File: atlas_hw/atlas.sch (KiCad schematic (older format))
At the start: 200 parts, among them J1 USB_C_Receptacle_USB2.0, J10 PSP_LCD, J2 DEBUG_STM, J3 PSP_TOUCH, J4 DEBUG_NRF, J5 CELL_THERM, J6 CELL_BARE, J7 AUX_THERM, J8 Micro_SD_Card_Det, J9 PSP_LCD_BL, Q1 Q_NMOS_DGS, Q2 Q_NMOS_DGS, Q3 Q_NMOS_DGS, Q4 Q_NMOS_DGS, Q5 Q_NMOS_DGS, SW1 SReset, SW2 Power, SW3 ResetSTM, SW4 ResetNRF, U1 STM32H723VITx, U10 BQ25611D, U11 STM6601CA2BDM6F, U12 BGA725L6, U13 LSF0108, U14 NPP600SNADJ, U15 TPS61073, U16 PAM2841, U17 NX3L1T3157, U2 W957A8MFYA5I, U3 MCP1811B, U4 TLV62569DBV, U5 nRF52810-QCxx, U6 LC709203F, U7 Teseo-LIV3F, U8 MS5637, U9 MC6470, Y1 16M, Y2 32k, Y3 32M, Y4 32k

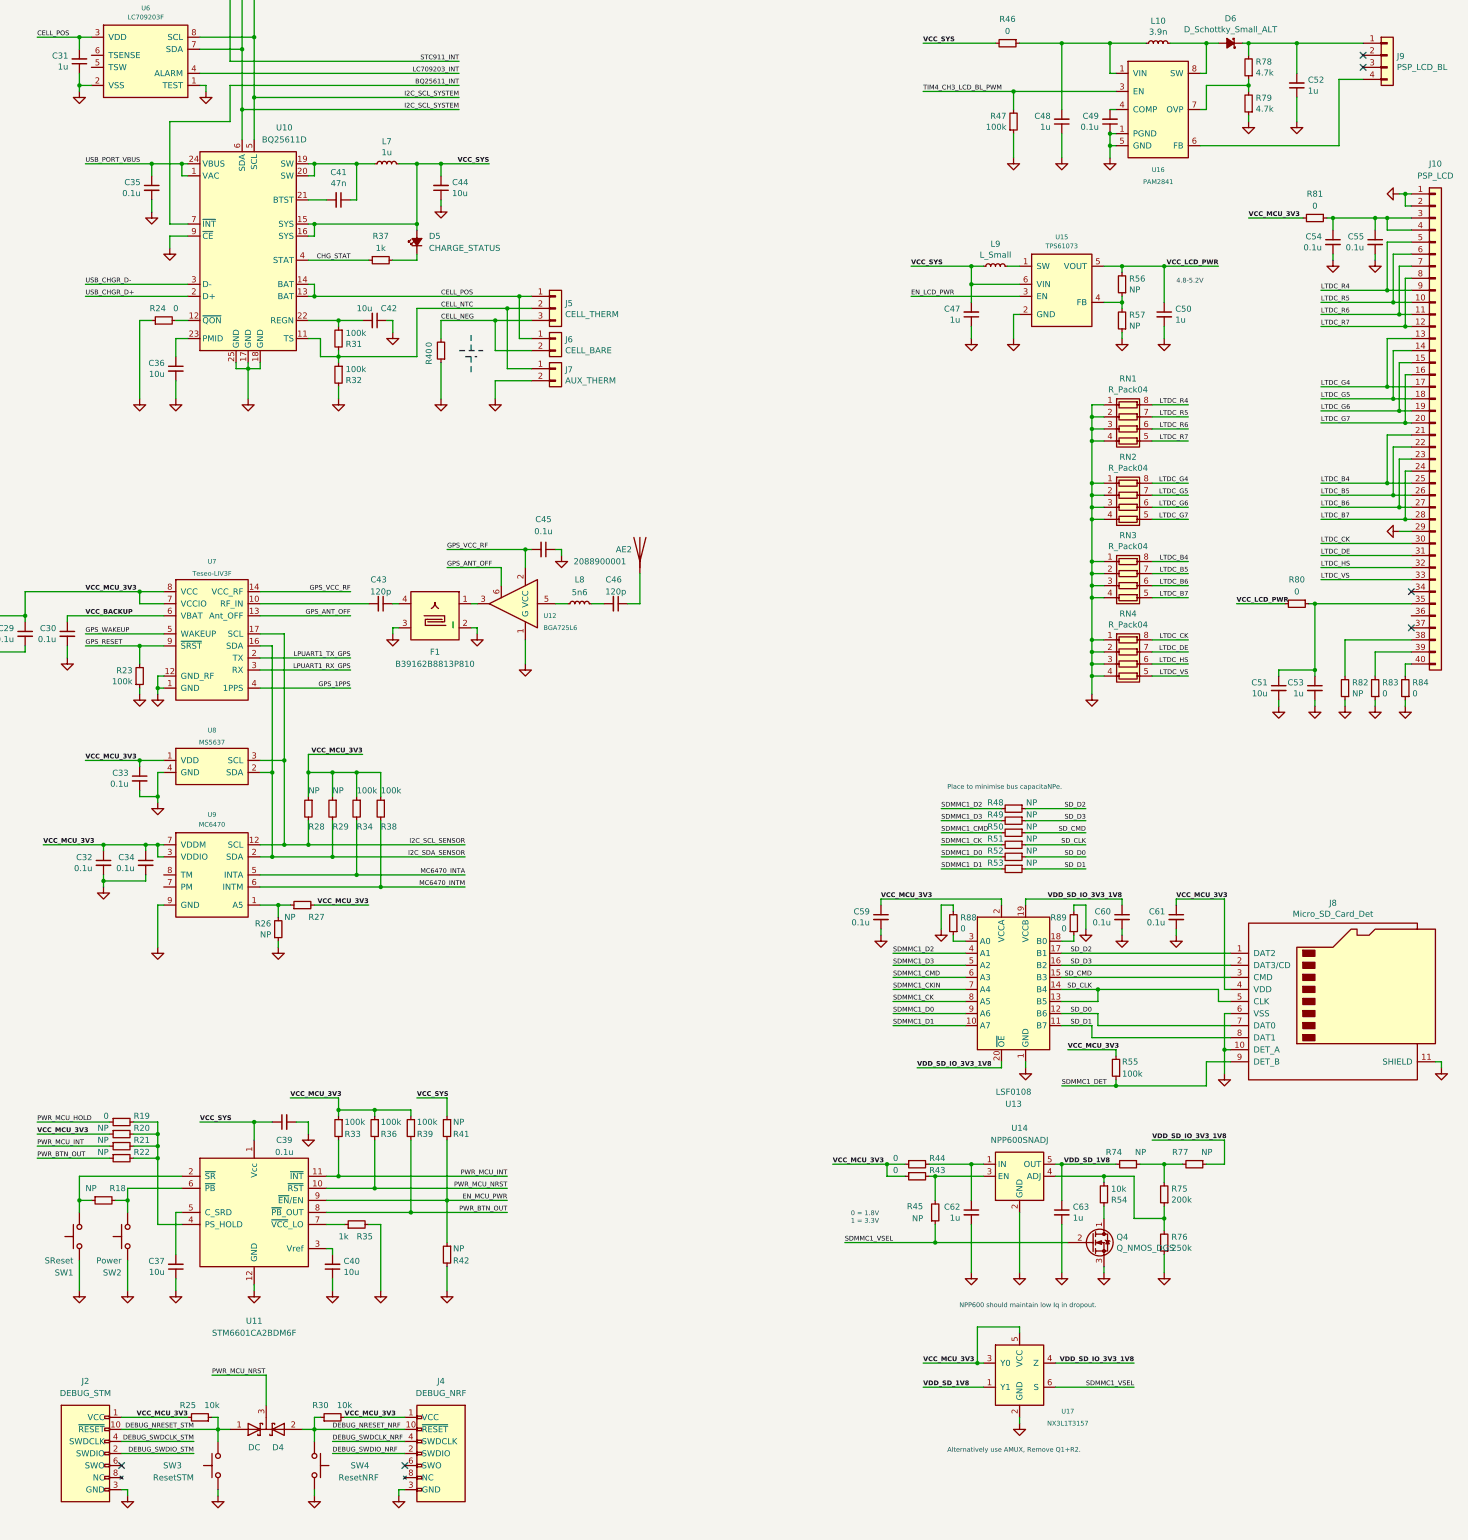
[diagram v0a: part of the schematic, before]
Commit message: started layout
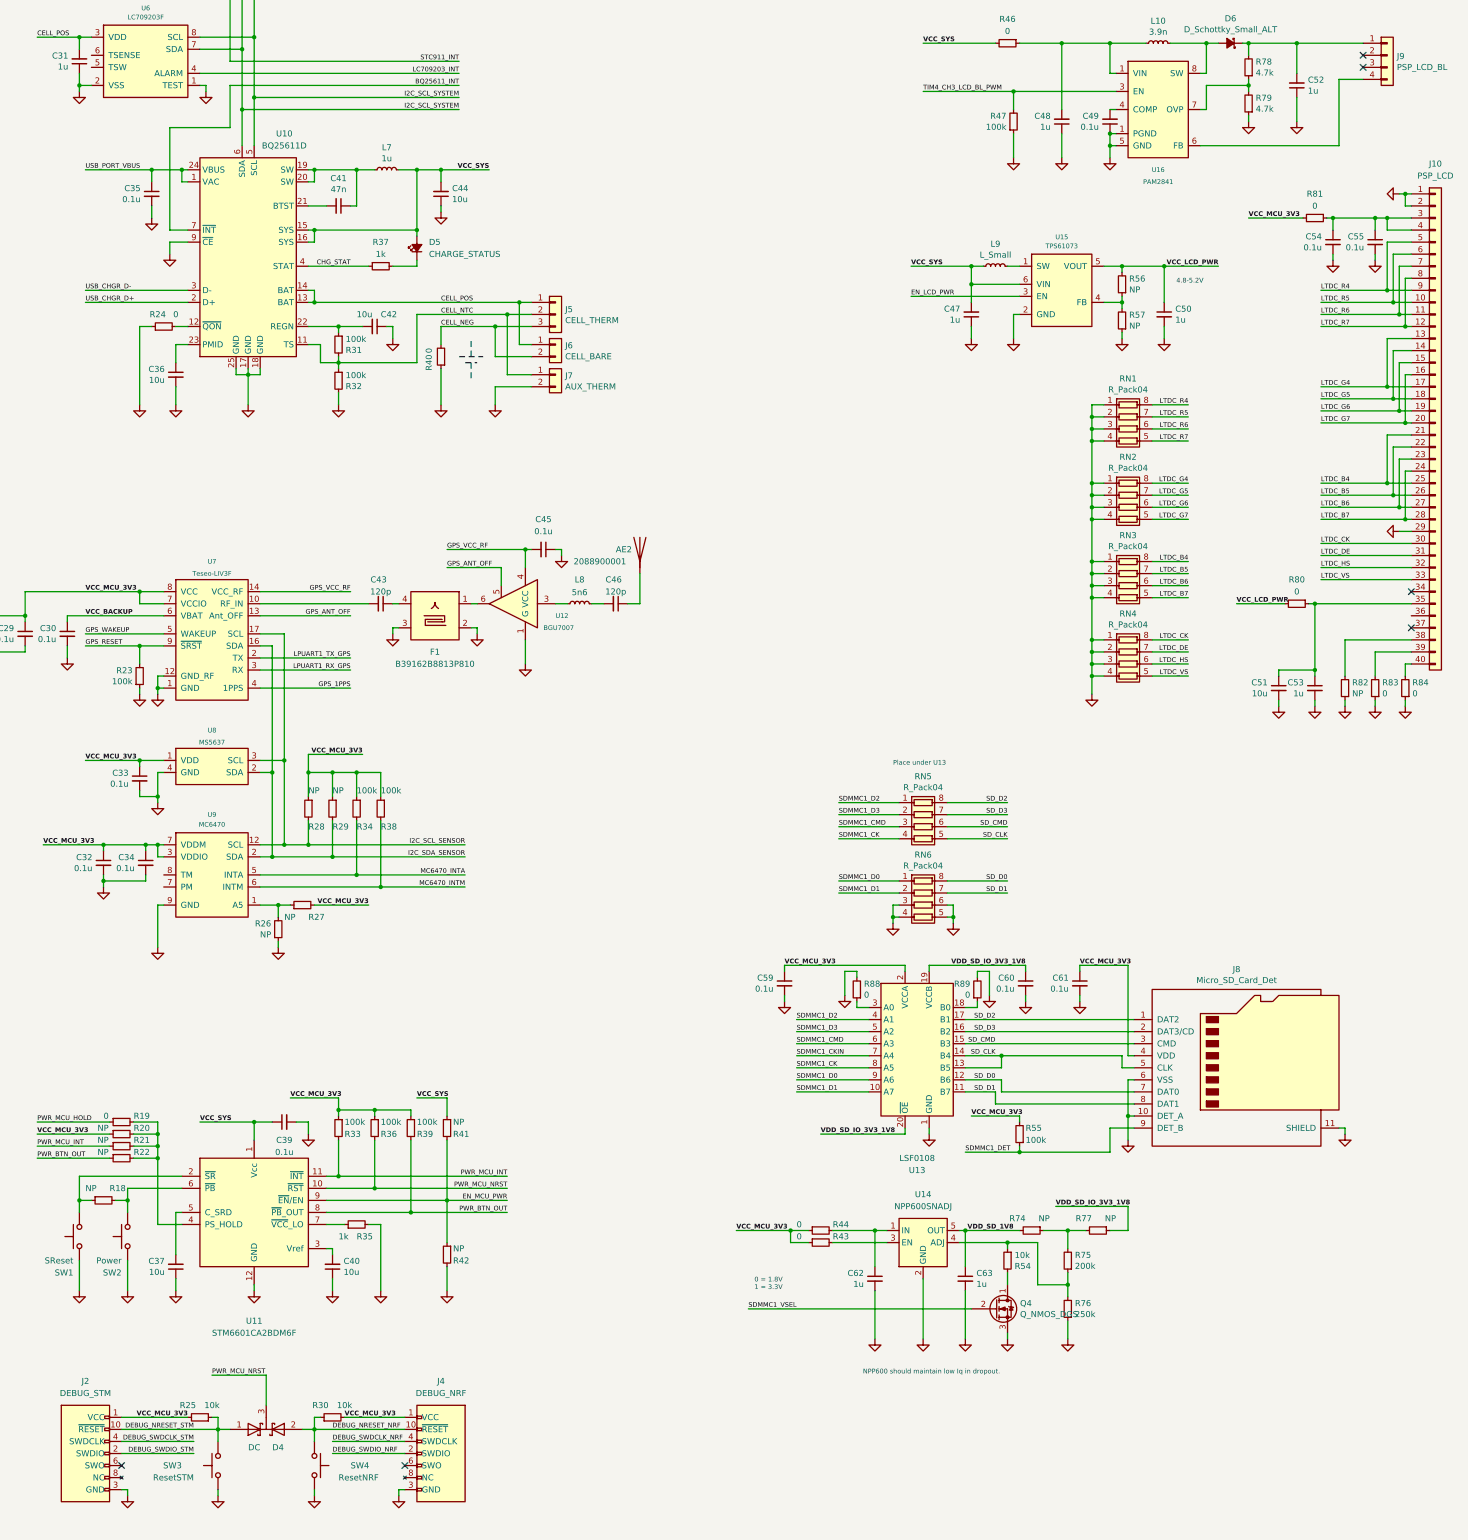
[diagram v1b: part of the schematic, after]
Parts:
- removed R45, R48, R49, R50, R51, R52, R53: NP, Resistor_SMD:R_0402_1005Metric, symbol Device:R_Small
- removed U12: BGA725L6, atlas:TSLP-6-2, symbol atlas:BGA725L6
- removed U17: NX3L1T3157, Package_TO_SOT_SMD:SOT-886, symbol atlas:NX3L1T3157
- added RN5, RN6: R_Pack04, Resistor_SMD:R_Array_Concave_4x0402, symbol Device:R_Pack04
- added U12: BGU7007, atlas:6-XSON_1.5x1.0mm_0.5mm, symbol atlas:BGU7007
- Y1, Y3: footprint Crystal:Crystal_SMD_2016-4Pin_2.0x1.6mm -> Crystal:Crystal_SMD_3225-4Pin_3.2x2.5mm
- Y2, Y4: footprint Crystal:Crystal_SMD_2012-2Pin_2.0x1.2mm -> Crystal:Crystal_SMD_3225-4Pin_3.2x2.5mm
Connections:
- net GND: now also RN6.3 (R3.1), RN6.4 (R4.1), RN6.5 (R4.2), RN6.6 (R3.2), U12.1 (G), U12.2 (G)
- net GPS_ANT_OFF: now also U12.5
- net GPS_VCC_RF: now also U12.4 (VCC)
- net SDMMC1_CK: now also RN5.4 (R4.1)
- net SDMMC1_CMD: now also RN5.3 (R3.1)
- net SDMMC1_D0: now also RN6.1 (R1.1)
- net SDMMC1_D1: now also RN6.2 (R2.1)
- net SDMMC1_D2: now also RN5.1 (R1.1)
- net SDMMC1_D3: now also RN5.2 (R2.1)
- net SD_CLK: now also RN5.5 (R4.2)
- net SD_CMD: now also RN5.6 (R3.2)
- net SD_D0: now also RN6.8 (R1.2)
- net SD_D1: now also RN6.7 (R2.2)
- net SD_D2: now also RN5.8 (R1.2)
- net SD_D3: now also RN5.7 (R2.2)
- net at F1.1: now also U12.6
- net at L8.1: now also U12.3
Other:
- note added: "Place under U13"
- note removed: "Alternatively use AMUX, Remove Q1+R2."
- note removed: "Place to minimise bus capacitaNPe."
- moved on the sheet: C35, C36, C41, C42, C44, C59, C60, C61, C62, C63, D5, J5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
